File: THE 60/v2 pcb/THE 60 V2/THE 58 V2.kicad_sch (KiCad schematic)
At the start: 136 parts, among them J1 Conn_01x02_Socket, J2 Conn_01x02_Socket, SW1 Switch, SW2 Switch, SW3 Switch, SW4 Switch, U1 Nice_Nano_V2, U2 Nice_Nano_V2, U3 TRRS, U4 TRRS

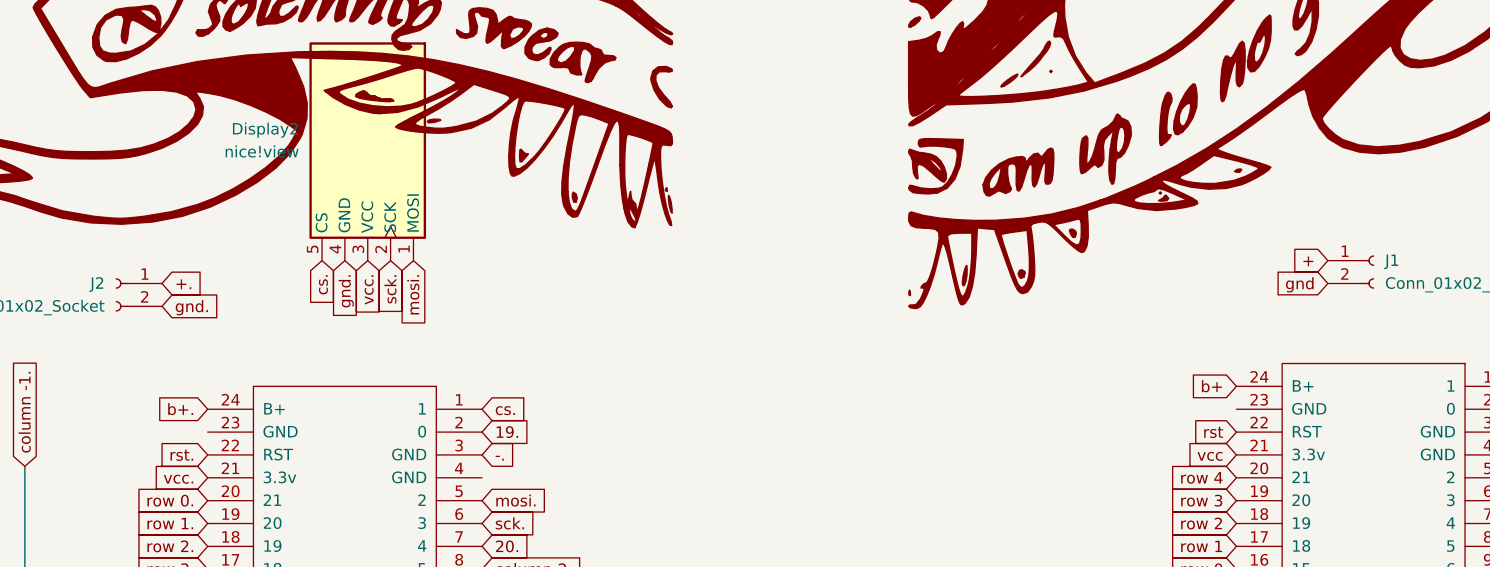
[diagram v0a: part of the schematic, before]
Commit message: z
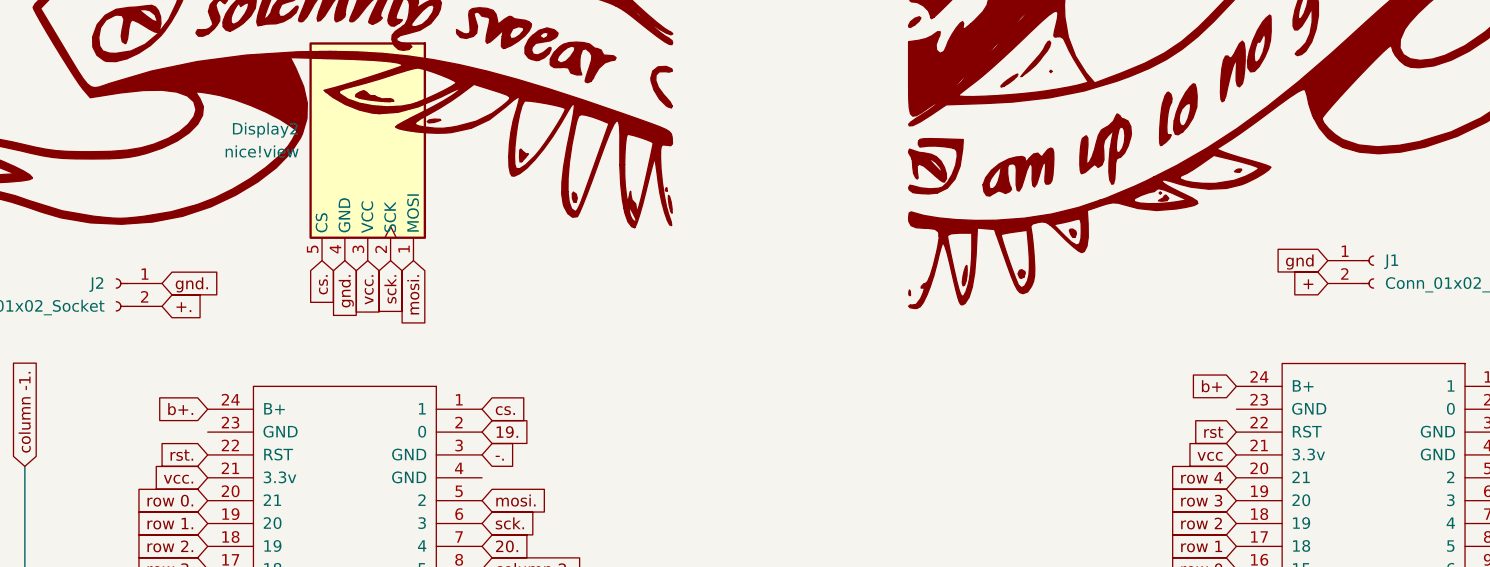
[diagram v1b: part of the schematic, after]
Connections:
- net +: now also J1.2 (Pin_2); no longer J1.1 (Pin_1)
- net +.: now also J2.2 (Pin_2); no longer J2.1 (Pin_1)
- net gnd: now also J1.1 (Pin_1); no longer J1.2 (Pin_2)
- net gnd.: now also J2.1 (Pin_1); no longer J2.2 (Pin_2)
